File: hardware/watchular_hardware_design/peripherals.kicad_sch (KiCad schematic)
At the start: 15 parts, among them Q1 BC817

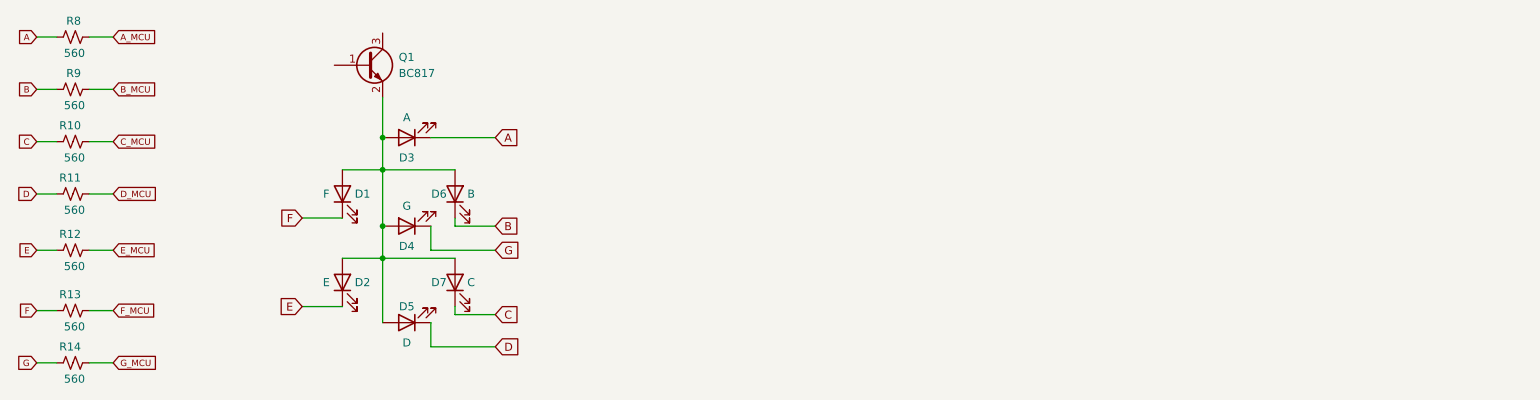
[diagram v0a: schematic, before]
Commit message: Added components for 4 digits.
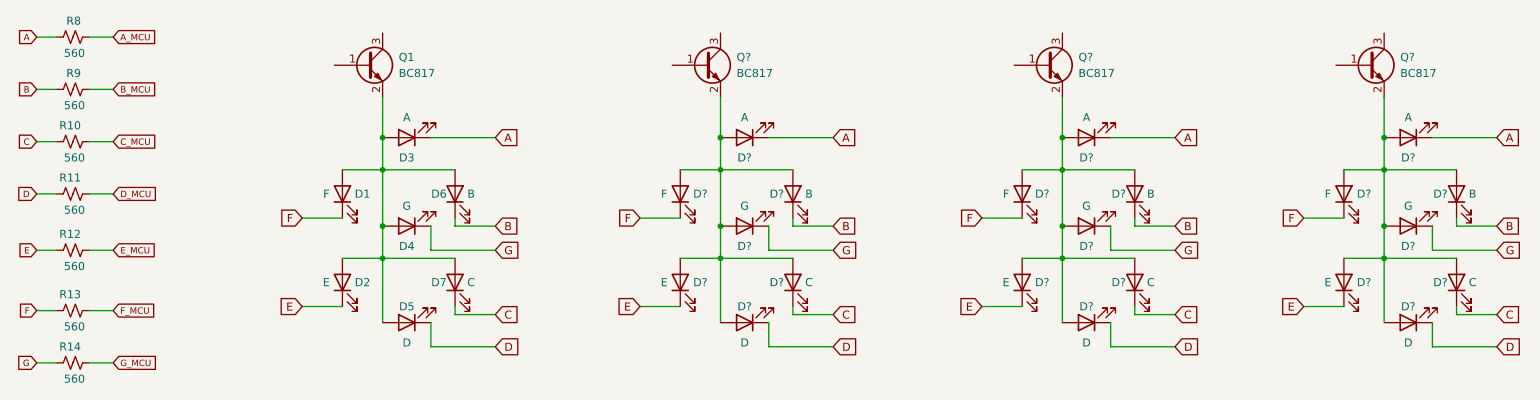
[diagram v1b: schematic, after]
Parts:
- added D? (x3): F, LED_SMD:LED_0603_1608Metric, symbol Device:LED
- added D? (x3): E, LED_SMD:LED_0603_1608Metric, symbol Device:LED
- added D? (x3): G, LED_SMD:LED_0603_1608Metric, symbol Device:LED
- added D? (x3): D, LED_SMD:LED_0603_1608Metric, symbol Device:LED
- added D? (x3): B, LED_SMD:LED_0603_1608Metric, symbol Device:LED
- added D? (x3): A, LED_SMD:LED_0603_1608Metric, symbol Device:LED
- added D? (x3): C, LED_SMD:LED_0603_1608Metric, symbol Device:LED
- added Q? (x3): BC817, Package_TO_SOT_SMD:SOT-23, symbol Transistor_BJT:BC817
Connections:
- net A: now also D?.1 (K), D?.1 (K), D?.1 (K)
- net B: now also D?.1 (K), D?.1 (K), D?.1 (K)
- net C: now also D?.1 (K), D?.1 (K), D?.1 (K)
- net D: now also D?.1 (K), D?.1 (K), D?.1 (K)
- net E: now also D?.1 (K), D?.1 (K), D?.1 (K)
- net F: now also D?.1 (K), D?.1 (K), D?.1 (K)
- net G: now also D?.1 (K), D?.1 (K), D?.1 (K)
- new net: D?.2 (A), D?.2 (A), D?.2 (A), D?.2 (A), D?.2 (A), D?.2 (A), D?.2 (A), Q?.2 (E) (x3)
